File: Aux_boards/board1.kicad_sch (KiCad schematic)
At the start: 9 parts, among them J1 DB25_Receptacle_MountingHoles, J4 DC37_Plug_MountingHoles, U2 AMS1117-3.3

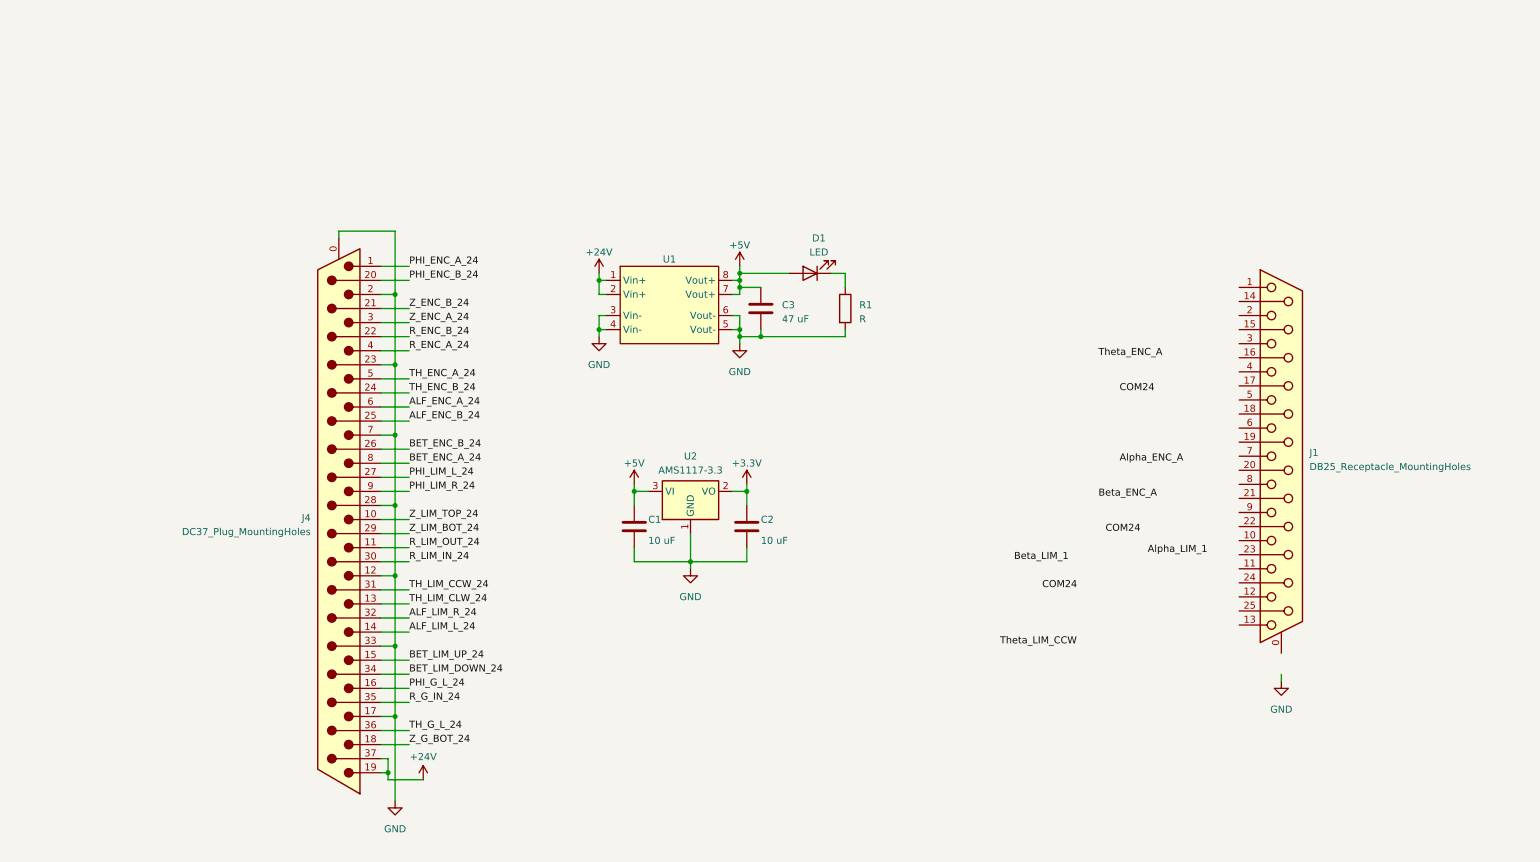
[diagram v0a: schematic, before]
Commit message: worked on auxboard_1
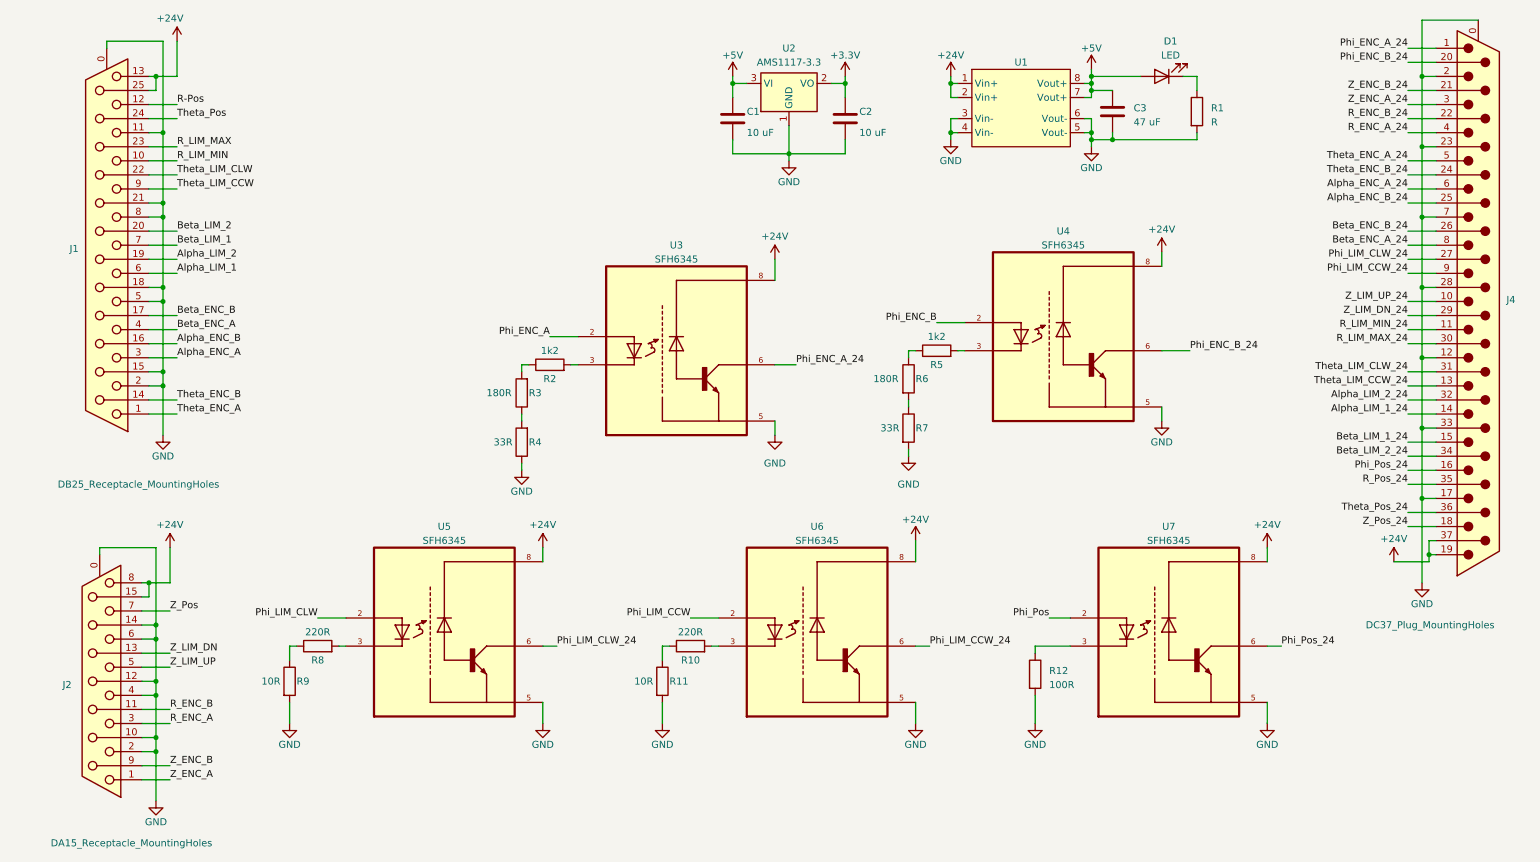
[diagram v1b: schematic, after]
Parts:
- added J2: DA15_Receptacle_MountingHoles, symbol Connector:DA15_Receptacle_MountingHoles
- added R10, R8: 220R, symbol Device:R
- added R11, R9: 10R, symbol Device:R
- added R12: 100R, symbol Device:R
- added R2, R5: 1k2, symbol Device:R
- added R3, R6: 180R, symbol Device:R
- added R4, R7: 33R, symbol Device:R
- added U3, U4, U5, U6, U7: SFH6345, SFH6345:SFH6345, symbol SFH6345:SFH6345
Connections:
- net +24V: now also J1.13, J1.25 (P25), J2.15 (P15), J2.8, U3.8, U4.8, U5.8, U6.8, U7.8
- net Alpha_ENC_A: now also J1.3
- net Alpha_LIM_1: now also J1.6
- net Beta_ENC_A: now also J1.4
- net Beta_LIM_1: now also J1.7
- net GND: now also J1.0 (PAD), J1.11, J1.15 (P15), J1.18 (P18), J1.2, J1.21 (P21), J1.5, J1.8, J2.0 (PAD), J2.10 (P10), J2.12 (P12), J2.14 (P14), J2.2, J2.4, J2.6, R11.2, R12.2, R4.1, R7.2, R9.2, U3.5, U4.5, U5.5, U6.5, U7.5
- net Theta_ENC_A: now also J1.1
- net Theta_LIM_CCW: now also J1.9
- net R_LIM_MIN: now reaches J1.10
- net R-Pos: now reaches J1.12
- net Theta_ENC_B: now reaches J1.14 (P14)
- net Alpha_ENC_B: now reaches J1.16 (P16)
- net Beta_ENC_B: now reaches J1.17 (P17)
- net Alpha_LIM_2: now reaches J1.19 (P19)
- net Beta_LIM_2: now reaches J1.20 (P20)
- net Theta_LIM_CLW: now reaches J1.22 (P22)
- net R_LIM_MAX: now reaches J1.23 (P23)
- net Theta_Pos: now reaches J1.24 (P24)
- net ALF_ENC_A_24 renamed Alpha_ENC_A_24
- net ALF_ENC_B_24 renamed Alpha_ENC_B_24
- net ALF_LIM_L_24 renamed Alpha_LIM_1_24
- net ALF_LIM_R_24 renamed Alpha_LIM_2_24
- net BET_ENC_A_24 renamed Beta_ENC_A_24
- net BET_ENC_B_24 renamed Beta_ENC_B_24
- net BET_LIM_DOWN_24 renamed Beta_LIM_2_24
- net BET_LIM_UP_24 renamed Beta_LIM_1_24
- net PHI_ENC_A_24 renamed Phi_ENC_A_24
- net Phi_ENC_A_24: now also U3.6
- net PHI_ENC_B_24 renamed Phi_ENC_B_24
- net Phi_ENC_B_24: now also U4.6
- net PHI_G_L_24 renamed Phi_Pos_24
- net Phi_Pos_24: now also U7.6
- net PHI_LIM_L_24 renamed Phi_LIM_CLW_24
- net Phi_LIM_CLW_24: now also U5.6
- net PHI_LIM_R_24 renamed Phi_LIM_CCW_24
- net Phi_LIM_CCW_24: now also U6.6
- net R_G_IN_24 renamed R_Pos_24
- net R_LIM_IN_24 renamed R_LIM_MAX_24
- net R_LIM_OUT_24 renamed R_LIM_MIN_24
- net TH_ENC_A_24 renamed Theta_ENC_A_24
- net TH_ENC_B_24 renamed Theta_ENC_B_24
- net TH_G_L_24 renamed Theta_Pos_24
- net TH_LIM_CCW_24 renamed Theta_LIM_CLW_24
- net TH_LIM_CLW_24 renamed Theta_LIM_CCW_24
- net Z_G_BOT_24 renamed Z_Pos_24
- net Z_LIM_BOT_24 renamed Z_LIM_DN_24
- net Z_LIM_TOP_24 renamed Z_LIM_UP_24
- new net: R5.1, R6.1
- new net: R5.2, U4.3
- new net: R2.1, R3.2
- new net: R2.2, U3.3
- new net: R10.1, R11.1
- new net: R10.2, U6.3
- new net: R12.1, U7.3
- new net: R6.2, R7.1
- new net: R8.1, R9.1
- new net: R3.1, R4.2
- new net: R8.2, U5.3
- new net Phi_ENC_A: U3.2
- new net Phi_ENC_B: U4.2
- new net Phi_LIM_CCW: U6.2
- new net Phi_LIM_CLW: U5.2
- new net Phi_Pos: U7.2
- new net R_ENC_A: J2.3
- new net R_ENC_B: J2.11 (P111)
- new net Z_ENC_A: J2.1
- new net Z_ENC_B: J2.9 (P9)
- new net Z_LIM_DN: J2.13 (P13)
- new net Z_LIM_UP: J2.5
- new net Z_Pos: J2.7
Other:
- moved on the sheet: C1, C2, C3, D1, J1, J4, R1, U1, U2
